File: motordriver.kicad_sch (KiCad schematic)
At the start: 40 parts, among them Q401 STP15810, Q402 STP15810, Q403 STP15810, Q404 STP15810, Q405 STP15810, Q406 STP15810, Q407 STP15810, Q408 STP15810, U401 LM5110-1MX, U402 LM5110-1MX, U403 LM5110-1MX, U404 LM5110-1MX

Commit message: Start PCB
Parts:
- R401, R402, R403, R404, R405, R406, R407, R408, R409, R410, R411, R412: footprint Resistor_SMD:R_0805_2012Metric_Pad1.20x1.40mm_HandSolder -> Resistor_SMD:R_0603_1608Metric_Pad0.98x0.95mm_HandSolder
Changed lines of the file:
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@@
       (effects (font (size 1.27 1.27)) (justify left))
     )
-    (property "Footprint" "Resistor_SMD:R_0805_2012Metric_Pad1.20x1.40mm_HandSolder" (id 2) (at 26.162 46.99 90)
+    (property "Footprint" "Resistor_SMD:R_0603_1608Metric_Pad0.98x0.95mm_HandSolder" (id 2) (at 26.162 46.99 90)
       (effects (font (size 1.27 1.27)) hide)
     )
@@
     (property "Reference" "R402" (id 0) (at 78.74 38.1 90))
     (property "Value" "4.7R" (id 1) (at 78.74 40.64 90))
-    (property "Footprint" "Resistor_SMD:R_0805_2012Metric_Pad1.20x1.40mm_HandSolder" (id 2) (at 78.74 42.418 90)
+    (property "Footprint" "Resistor_SMD:R_0603_1608Metric_Pad0.98x0.95mm_HandSolder" (id 2) (at 78.74 42.418 90)
       (effects (font (size 1.27 1.27)) hide)
     )
@@
     (property "Reference" "R403" (id 0) (at 78.74 45.72 90))
     (property "Value" "4.7R" (id 1) (at 78.74 43.18 90))
-    (property "Footprint" "Resistor_SMD:R_0805_2012Metric_Pad1.20x1.40mm_HandSolder" (id 2) (at 78.74 41.402 90)
+    (property "Footprint" "Resistor_SMD:R_0603_1608Metric_Pad0.98x0.95mm_HandSolder" (id 2) (at 78.74 41.402 90)
       (effects (font (size 1.27 1.27)) hide)
     )
@@
     (property "Reference" "R404" (id 0) (at 78.74 95.25 90))
     (property "Value" "4.7R" (id 1) (at 78.74 97.79 90))
-    (property "Footprint" "Resistor_SMD:R_0805_2012Metric_Pad1.20x1.40mm_HandSolder" (id 2) (at 78.74 99.568 90)
+    (property "Footprint" "Resistor_SMD:R_0603_1608Metric_Pad0.98x0.95mm_HandSolder" (id 2) (at 78.74 99.568 90)
       (effects (font (size 1.27 1.27)) hide)
     )
@@
     (property "Reference" "R405" (id 0) (at 78.74 102.87 90))
     (property "Value" "4.7R" (id 1) (at 78.74 100.33 90))
-    (property "Footprint" "Resistor_SMD:R_0805_2012Metric_Pad1.20x1.40mm_HandSolder" (id 2) (at 78.74 98.552 90)
+    (property "Footprint" "Resistor_SMD:R_0603_1608Metric_Pad0.98x0.95mm_HandSolder" (id 2) (at 78.74 98.552 90)
       (effects (font (size 1.27 1.27)) hide)
     )
@@
       (effects (font (size 1.27 1.27)) (justify left))
     )
-    (property "Footprint" "Resistor_SMD:R_0805_2012Metric_Pad1.20x1.40mm_HandSolder" (id 2) (at 90.932 171.45 90)
+    (property "Footprint" "Resistor_SMD:R_0603_1608Metric_Pad0.98x0.95mm_HandSolder" (id 2) (at 90.932 171.45 90)
       (effects (font (size 1.27 1.27)) hide)
     )
@@
       (effects (font (size 1.27 1.27)) (justify left))
     )
-    (property "Footprint" "Resistor_SMD:R_0805_2012Metric_Pad1.20x1.40mm_HandSolder" (id 2) (at 127.762 171.45 90)
+    (property "Footprint" "Resistor_SMD:R_0603_1608Metric_Pad0.98x0.95mm_HandSolder" (id 2) (at 127.762 171.45 90)
       (effects (font (size 1.27 1.27)) hide)
     )
@@
       (effects (font (size 1.27 1.27)) (justify left))
     )
-    (property "Footprint" "Resistor_SMD:R_0805_2012Metric_Pad1.20x1.40mm_HandSolder" (id 2) (at 156.972 46.99 90)
+    (property "Footprint" "Resistor_SMD:R_0603_1608Metric_Pad0.98x0.95mm_HandSolder" (id 2) (at 156.972 46.99 90)
       (effects (font (size 1.27 1.27)) hide)
     )
@@
     (property "Reference" "R409" (id 0) (at 209.55 38.1 90))
     (property "Value" "4.7R" (id 1) (at 209.55 40.64 90))
-    (property "Footprint" "Resistor_SMD:R_0805_2012Metric_Pad1.20x1.40mm_HandSolder" (id 2) (at 209.55 42.418 90)
+    (property "Footprint" "Resistor_SMD:R_0603_1608Metric_Pad0.98x0.95mm_HandSolder" (id 2) (at 209.55 42.418 90)
       (effects (font (size 1.27 1.27)) hide)
     )
@@
     (property "Reference" "R410" (id 0) (at 209.55 45.72 90))
     (property "Value" "4.7R" (id 1) (at 209.55 43.18 90))
-    (property "Footprint" "Resistor_SMD:R_0805_2012Metric_Pad1.20x1.40mm_HandSolder" (id 2) (at 209.55 41.402 90)
+    (property "Footprint" "Resistor_SMD:R_0603_1608Metric_Pad0.98x0.95mm_HandSolder" (id 2) (at 209.55 41.402 90)
       (effects (font (size 1.27 1.27)) hide)
     )
@@
     (property "Reference" "R411" (id 0) (at 209.55 95.25 90))
     (property "Value" "4.7R" (id 1) (at 209.55 97.79 90))
-    (property "Footprint" "Resistor_SMD:R_0805_2012Metric_Pad1.20x1.40mm_HandSolder" (id 2) (at 209.55 99.568 90)
+    (property "Footprint" "Resistor_SMD:R_0603_1608Metric_Pad0.98x0.95mm_HandSolder" (id 2) (at 209.55 99.568 90)
       (effects (font (size 1.27 1.27)) hide)
     )
@@
     (property "Reference" "R412" (id 0) (at 209.55 102.87 90))
     (property "Value" "4.7R" (id 1) (at 209.55 100.33 90))
-    (property "Footprint" "Resistor_SMD:R_0805_2012Metric_Pad1.20x1.40mm_HandSolder" (id 2) (at 209.55 98.552 90)
+    (property "Footprint" "Resistor_SMD:R_0603_1608Metric_Pad0.98x0.95mm_HandSolder" (id 2) (at 209.55 98.552 90)
       (effects (font (size 1.27 1.27)) hide)
     )

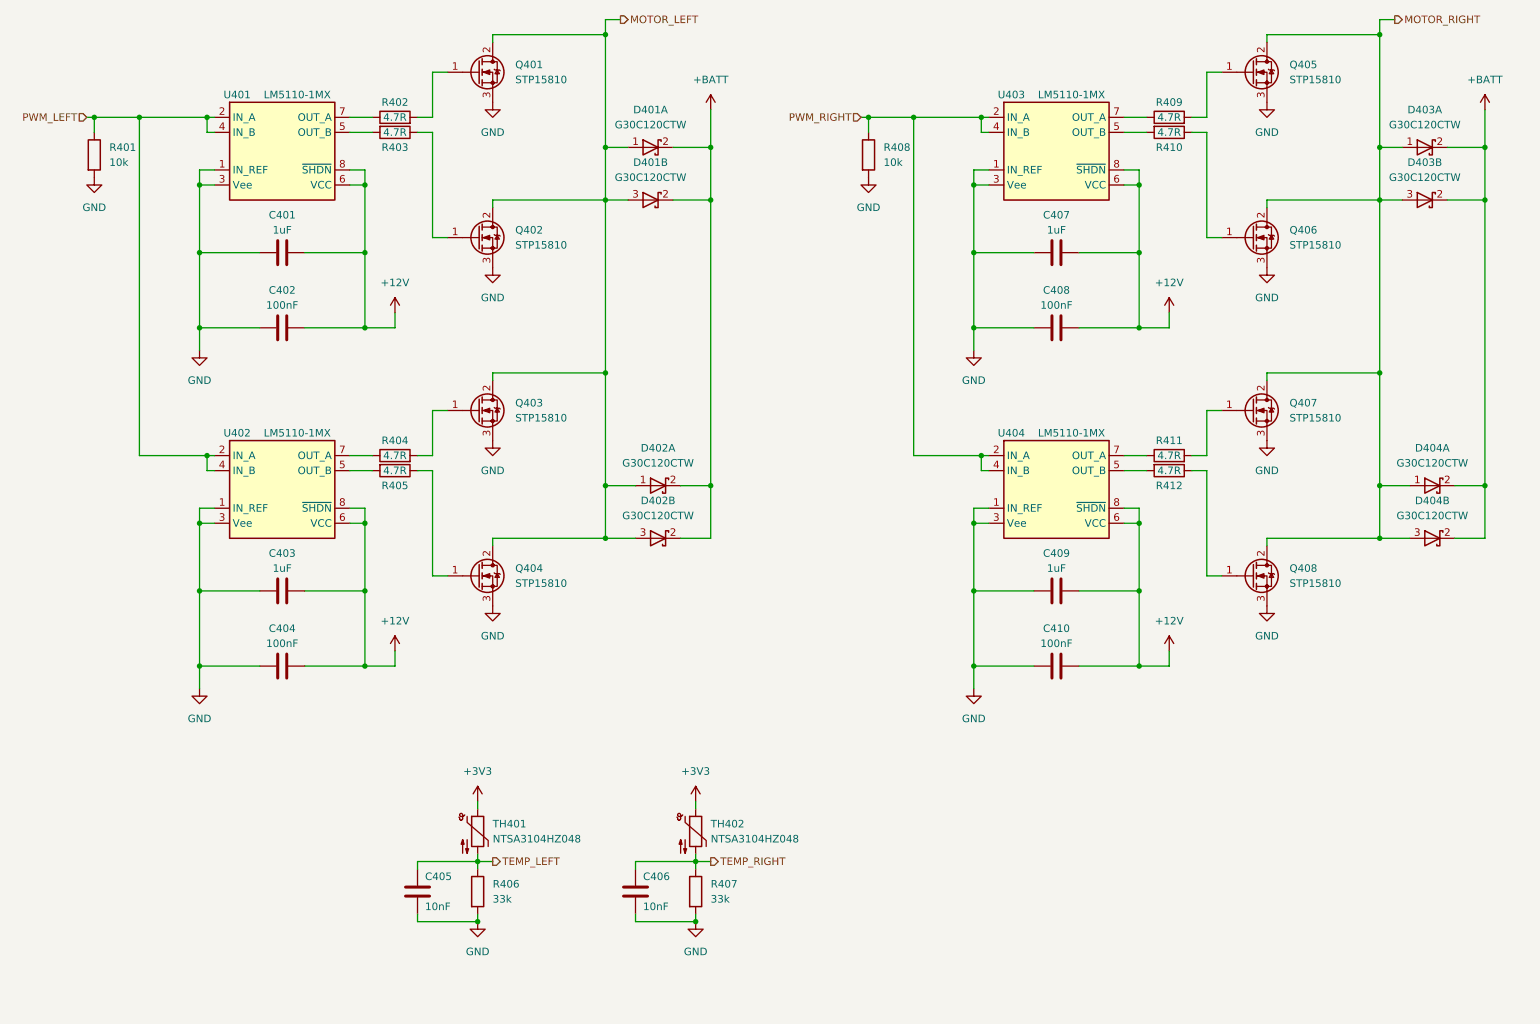
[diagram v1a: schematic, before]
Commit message: First PCB commit
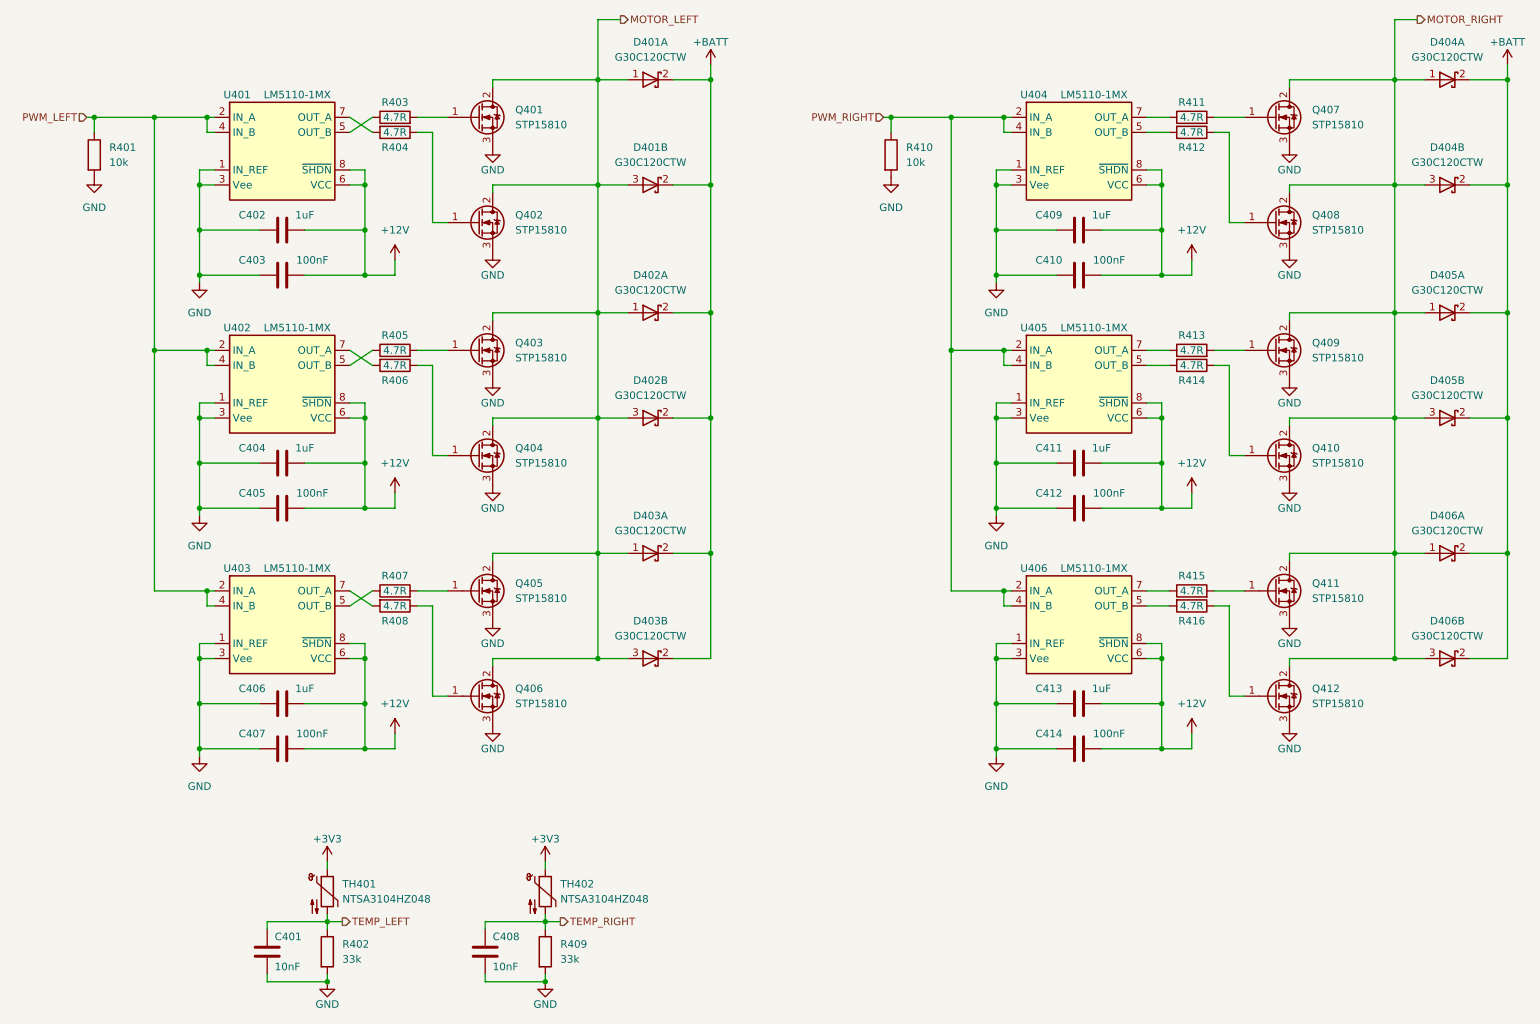
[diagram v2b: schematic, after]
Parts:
- removed C403: 1uF, Capacitor_SMD:C_0805_2012Metric_Pad1.18x1.45mm_HandSolder, symbol Device:C
- removed C408: 100nF, Capacitor_SMD:C_0805_2012Metric_Pad1.18x1.45mm_HandSolder, symbol Device:C
- removed R404, R409: 4.7R, Resistor_SMD:R_0603_1608Metric_Pad0.98x0.95mm_HandSolder, symbol Device:R
- added C405, C412, C414: 100nF, Capacitor_SMD:C_0603_1608Metric_Pad1.08x0.95mm_HandSolder, symbol Device:C
- added C406, C411, C413: 1uF, Capacitor_SMD:C_0603_1608Metric_Pad1.08x0.95mm_HandSolder, symbol Device:C
- added D405, D406: G30C120CTW, Package_TO_SOT_THT:TO-220-3_Vertical, symbol GozLib:G30C120CTW
- added Q409, Q410, Q411, Q412: STP15810, Package_TO_SOT_THT:TO-220-3_Vertical, symbol GozLib:STP15810
- added R406, R407, R413, R414, R415, R416: 4.7R, Resistor_SMD:R_0603_1608Metric_Pad0.98x0.95mm_HandSolder, symbol Device:R
- added U405, U406: LM5110-1MX, Package_SO:SOIC-8_3.9x4.9mm_P1.27mm, symbol GozLib:LM5110-1MX
- C401: renamed from C405; footprint Capacitor_SMD:C_0805_2012Metric_Pad1.18x1.45mm_HandSolder -> Capacitor_SMD:C_0603_1608Metric_Pad1.08x0.95mm_HandSolder
- C402: renamed from C401; footprint Capacitor_SMD:C_0805_2012Metric_Pad1.18x1.45mm_HandSolder -> Capacitor_SMD:C_0603_1608Metric_Pad1.08x0.95mm_HandSolder
- C403: renamed from C402; footprint Capacitor_SMD:C_0805_2012Metric_Pad1.18x1.45mm_HandSolder -> Capacitor_SMD:C_0603_1608Metric_Pad1.08x0.95mm_HandSolder
- C404: value 100nF -> 1uF; footprint Capacitor_SMD:C_0805_2012Metric_Pad1.18x1.45mm_HandSolder -> Capacitor_SMD:C_0603_1608Metric_Pad1.08x0.95mm_HandSolder
- C407: value 1uF -> 100nF; footprint Capacitor_SMD:C_0805_2012Metric_Pad1.18x1.45mm_HandSolder -> Capacitor_SMD:C_0603_1608Metric_Pad1.08x0.95mm_HandSolder
- C408: renamed from C406; footprint Capacitor_SMD:C_0805_2012Metric_Pad1.18x1.45mm_HandSolder -> Capacitor_SMD:C_0603_1608Metric_Pad1.08x0.95mm_HandSolder
- C409, C410: footprint Capacitor_SMD:C_0805_2012Metric_Pad1.18x1.45mm_HandSolder -> Capacitor_SMD:C_0603_1608Metric_Pad1.08x0.95mm_HandSolder
- R408: value 10k -> 4.7R
- R410: value 4.7R -> 10k
- renumbered R406 to R402, R402 to R403, R403 to R404, R407 to R409
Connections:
- net +12V: now also C405.2, C406.2, C411.2, C412.2, C413.2, C414.2, U405.6 (VCC), U405.8 (~{SHDN}), U406.6 (VCC), U406.8 (~{SHDN})
- net +BATT: now also D405.2 (K), D405.2 (K), D406.2 (K), D406.2 (K)
- net GND: now also R410.2, C405.1, C406.1, C411.1, C412.1, C413.1, C414.1, Q409.3 (S), Q410.3 (S), Q411.3 (S), Q412.3 (S), U405.1 (IN_REF), U405.3 (Vee), U406.1 (IN_REF), U406.3 (Vee); no longer R408.2
- net MOTOR_LEFT: now also D403.1 (A), D403.3 (K), Q405.2 (D), Q406.2 (D)
- net MOTOR_RIGHT: now also D405.1 (A), D405.3 (K), D406.1 (A), D406.3 (K), Q409.2 (D), Q410.2 (D), Q411.2 (D), Q412.2 (D); no longer D403.1 (A), D403.3 (K), Q405.2 (D), Q406.2 (D)
- net PWM_LEFT: now also U403.2 (IN_A), U403.4 (IN_B)
- net PWM_RIGHT: now also R410.1, U405.2 (IN_A), U405.4 (IN_B), U406.2 (IN_A), U406.4 (IN_B); no longer R408.1, U403.2 (IN_A), U403.4 (IN_B)
- net at R404.2: now also U401.7 (OUT_A); no longer U401.5 (OUT_B)
- net at R403.1: now also U401.5 (OUT_B); no longer U401.7 (OUT_A)
- net at Q406.1 (G): now also R408.1; no longer R410.1
- net at U403.5 (OUT_B): now also R407.1; no longer R410.2
- net at U403.7 (OUT_A): now also R408.2
- net at Q405.1 (G): now also R407.2
- net at R405.1: now also U402.5 (OUT_B); no longer Q404.1 (G)
- net at R405.2: now also Q403.1 (G); no longer U402.5 (OUT_B)
- net at U402.7 (OUT_A): now also R406.2
- new net: R414.2, U405.5 (OUT_B)
- new net: R413.1, U405.7 (OUT_A)
- new net: Q410.1 (G), R414.1
- new net: Q412.1 (G), R416.1
- new net: Q404.1 (G), R406.1
- new net: R416.2, U406.5 (OUT_B)
- new net: R415.1, U406.7 (OUT_A)
- new net: Q409.1 (G), R413.2
- new net: Q411.1 (G), R415.2
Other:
- moved on the sheet: C401, C402, C403, C408, D401A, D401B, Q401, Q402, R402, R409, TH401, TH402
